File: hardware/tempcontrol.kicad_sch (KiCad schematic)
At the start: 17 parts, among them J10 FAN2, J9 FAN1, U12 EMC2305-x-AP

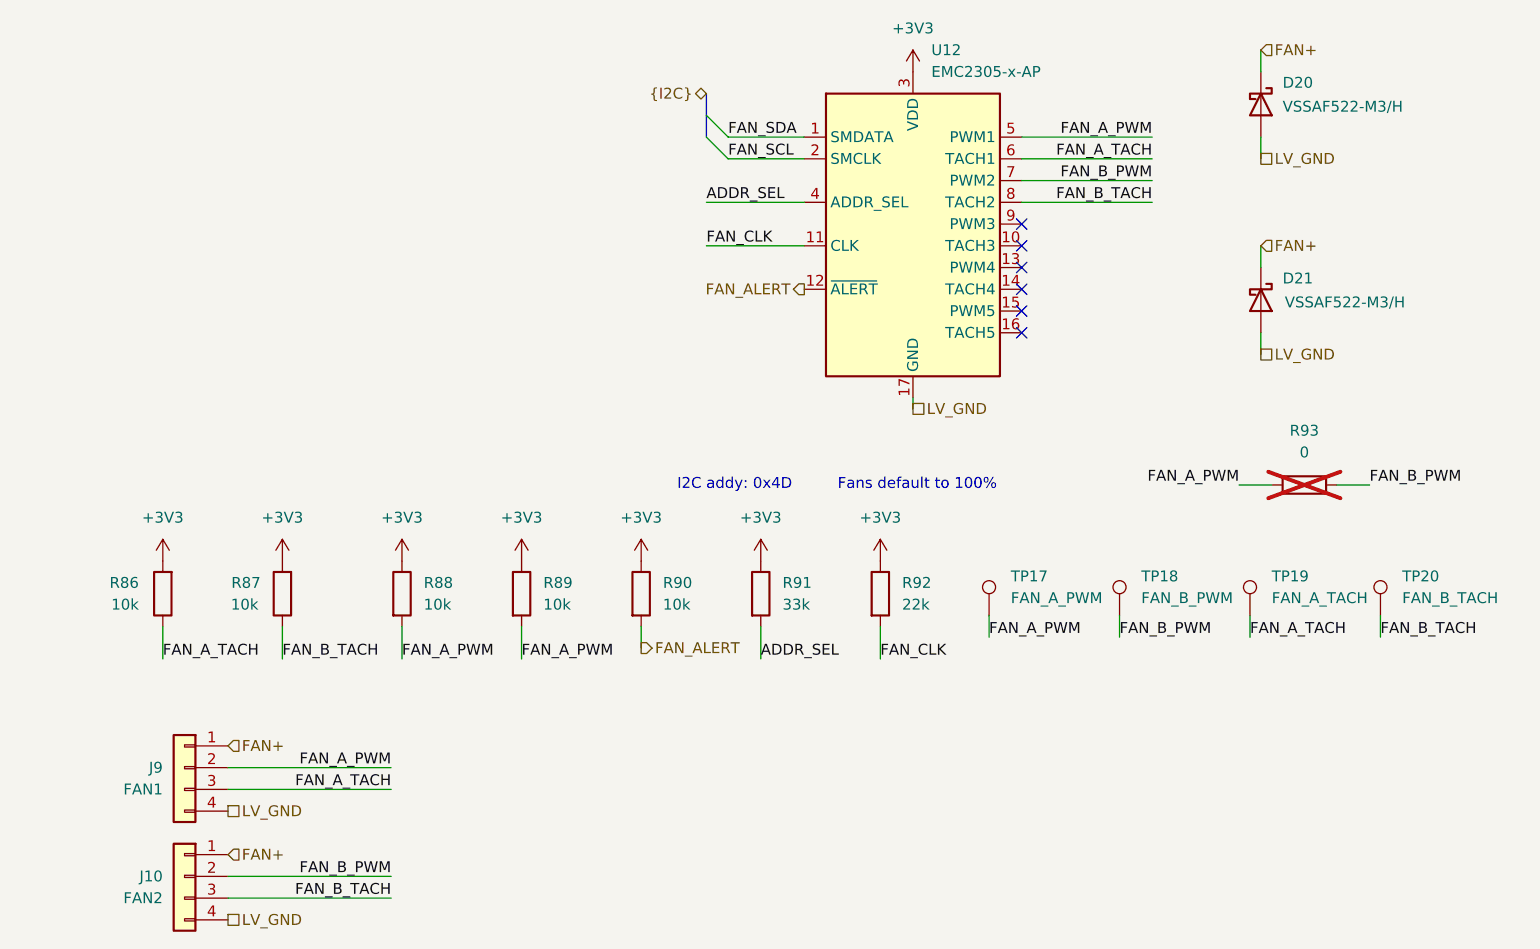
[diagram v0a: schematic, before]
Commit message: most reviews addressed oops
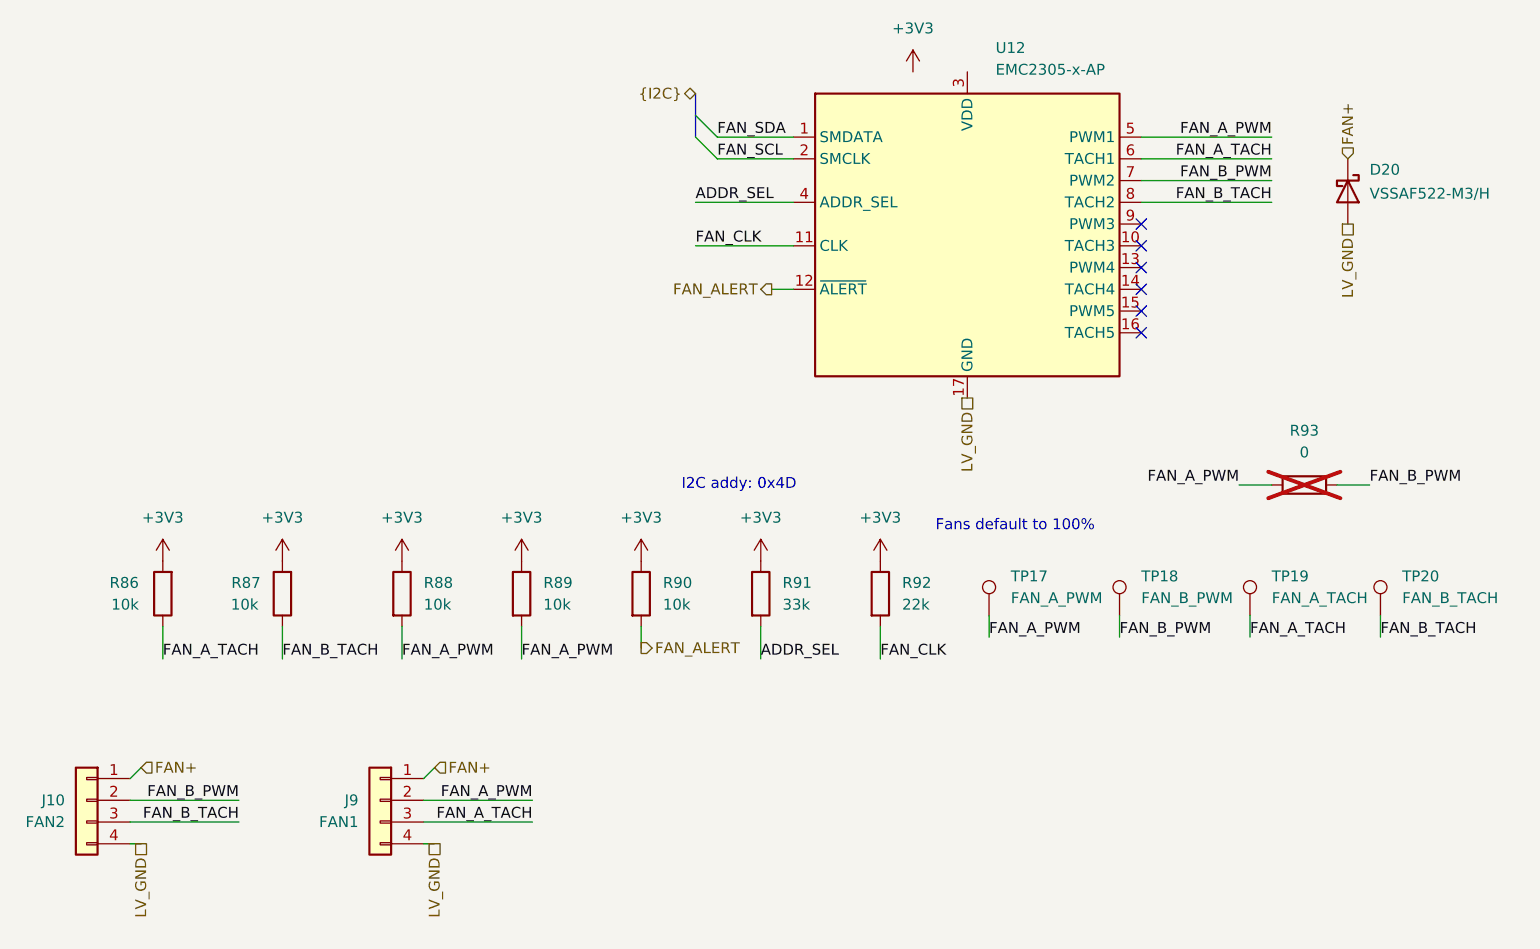
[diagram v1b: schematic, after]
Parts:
- removed D21: VSSAF522-M3/H, UTSVT_Passive:SODFL5026X125N, symbol Diode:C3D25170H
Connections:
- net +3V3: no longer U12.3 (VDD)
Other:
- moved on the sheet: D20, J10, J9, U12
